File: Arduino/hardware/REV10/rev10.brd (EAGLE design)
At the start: 98.3 x 55.9 mm, 48 parts, among them IC2 ATMEGA168-AU, Q1 32768Hz, U1 TC1185SMD, U2 ARDUINO

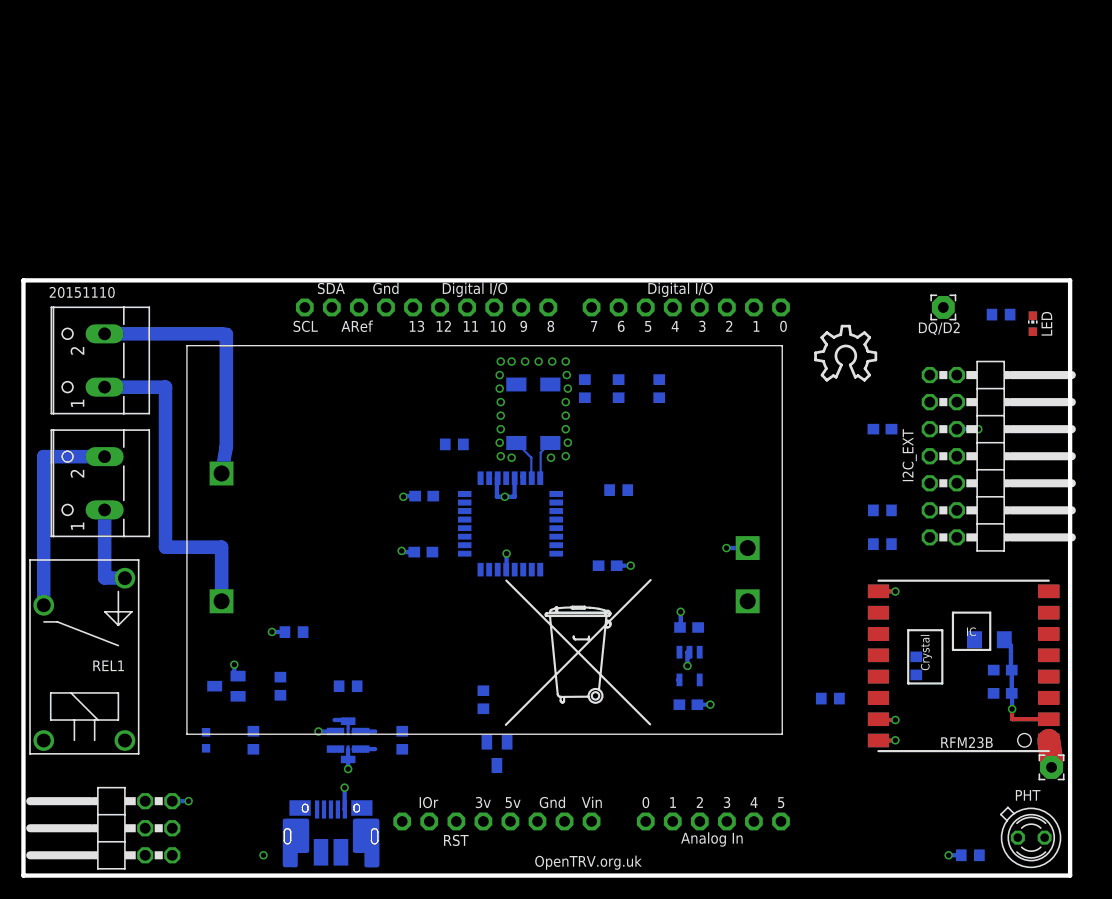
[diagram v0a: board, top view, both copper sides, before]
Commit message: rev10 reworked as per marks instruction. Almost ready for eyeball
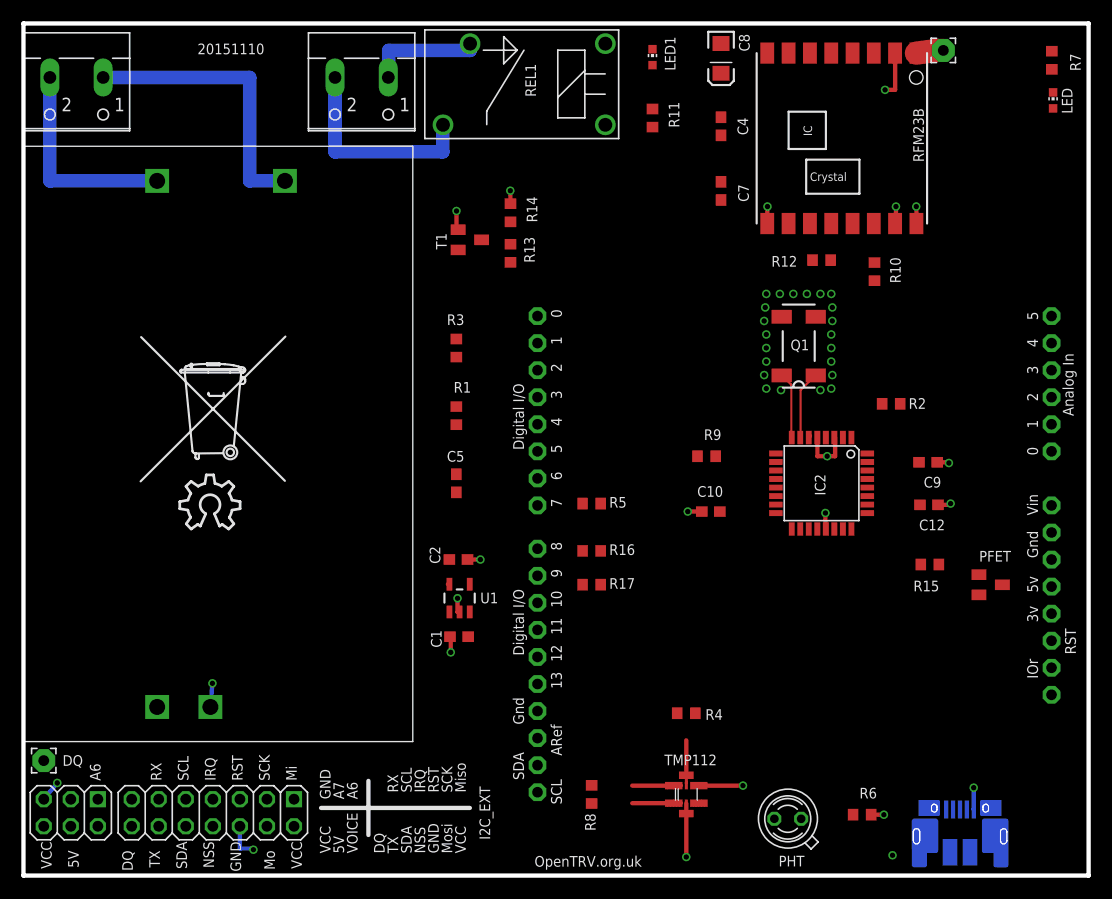
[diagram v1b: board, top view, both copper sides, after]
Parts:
- removed DQ/D2: (no value), wirepad:2,15/1,0
- added DQ: (no value), wirepad:2,15/1,0
- I2C_EXT: device pinhead:2X07/90 -> pinhead:2X07
- JP2: device pinhead:2X03/90 -> pinhead:2X03
- moved U2 85.1 mm to (101.6, -2.08), turned to 90 degrees
- moved REL1 81.5 mm to (55.9, 79.4), turned to 180 degrees
- moved I2C_EXT 80.9 mm to (17.8, 5.90), turned to 180 degrees
- moved LED1 76.6 mm to (59.1, 76.8), flipped to the top
- moved R11 69.4 mm to (59.1, 71.1), flipped to the top, turned to 270 degrees
- moved ANT1 68.1 mm to (86.4, 77.5), turned to 0 degrees
- moved U$1 61.3 mm to (14.7, 32.5)
- moved C8 60.1 mm to (65.5, 76.7), flipped to the top, turned to 270 degrees
- moved USBPOWER 59.1 mm to (90.5, 3.70)
- moved C4 57.5 mm to (65.5, 70.3), flipped to the top, turned to 270 degrees
- moved C7 54.1 mm to (65.5, 64.3), flipped to the top, turned to 270 degrees
- moved PSU 53.4 mm to (3.31, 68.6), turned to 270 degrees
- moved RFM23B 50.8 mm to (76.8, 69.2), turned to 270 degrees
- moved PFET 49.0 mm to (90.8, 27.3), flipped to the top, turned to 270 degrees
- moved T1 47.7 mm to (41.9, 59.7), flipped to the top
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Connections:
- removed net N$24: REL1.S, X3.1
- new net N$21: REL1.C, X3.1
- net D2: now also DQ.1; no longer DQ/D2.1
- net N$22: now also REL1.S; no longer REL1.C
- net N$4: now also X1.1; no longer X1.2
- net N$8: now also X1.2; no longer X1.1
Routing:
- net N$8: track 31.1 -> 19.8 mm
- net N$21: track 0.00 -> 10.9 mm
- net N$24: track 8.31 -> 0.00 mm
- net XTAL2: track 3.70 -> 6.24 mm
- net SDA: track 2.04 -> 4.58 mm
- net XTAL1: track 3.92 -> 6.46 mm
- net SCL: track 2.16 -> 4.58 mm
- net N$4: track 24.5 -> 26.8 mm
- net VCC: track 2.83 -> 4.73 mm
- net GND: track 47.5 -> 48.6 mm
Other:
- board size 98.3 x 55.9 mm -> 100 x 80 mm
- board text added: "5V"
- board text added: "A6"
- board text added: "A7"
- board text added: "DQ"
- board text added: "GND"
- board text added: "IRQ"
- board text added: "Mi"
- board text added: "Miso"
- board text added: "Mo"
- board text added: "Mosi"
- board text added: "NSS"
- board text added: "RST"
- board text added: "RX"
- board text added: "SCK"
- board text added: "SCL"
- board text added: "SDA"
- board text added: "TX"
- board text added: "VCC"
- board text added: "VOICE"
